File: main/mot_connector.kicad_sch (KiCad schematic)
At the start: 1 part, among them J1801 Conn_02x08_Odd_Even

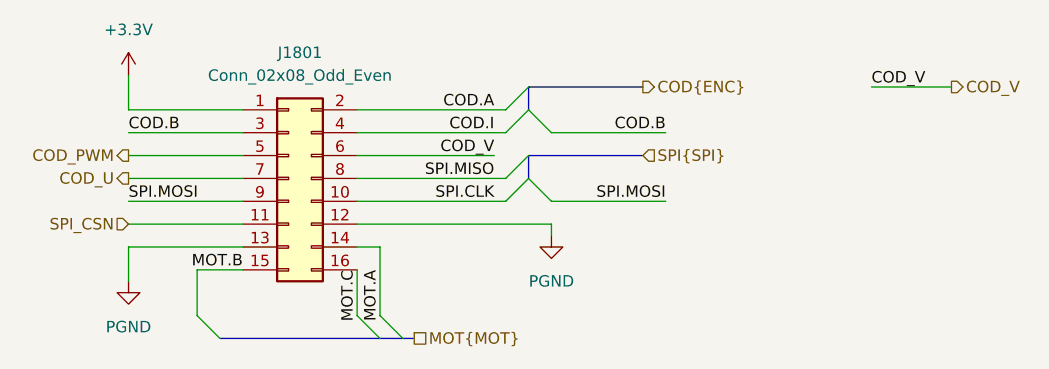
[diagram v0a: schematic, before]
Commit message: Revised with BOM ordered
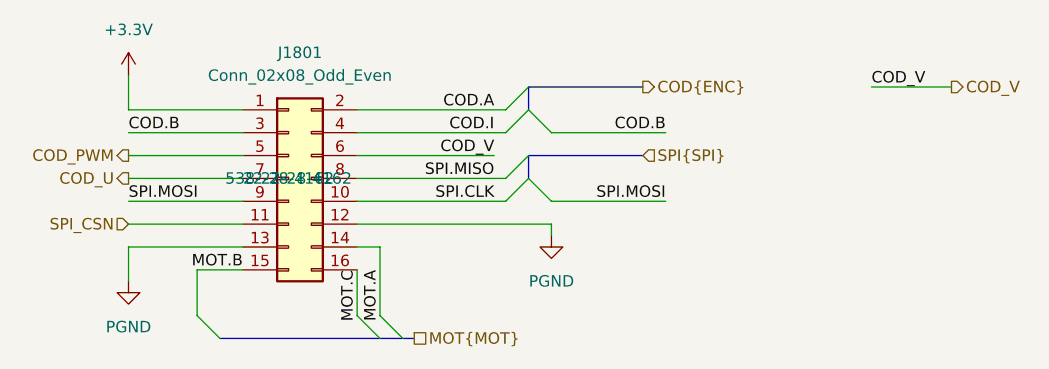
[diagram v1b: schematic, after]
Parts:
- J1801: MPN (none) -> 22-28-4162; Mouser SKU (none) -> 538-22-28-4162
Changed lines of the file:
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@@
+			)
+		)
+		(property "MPN" "22-28-4162 "
+			(at 146.05 76.2 0)
+			(effects
+				(font
+					(size 1.27 1.27)
+				)
+			)
+		)
+		(property "Mouser SKU" " 538-22-28-4162 "
+			(at 146.05 76.2 0)
+			(effects
+				(font
+					(size 1.27 1.27)
+				)
 			)
 		)
